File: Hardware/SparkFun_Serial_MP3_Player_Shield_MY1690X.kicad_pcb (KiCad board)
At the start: 2 copper layers, 53.3 x 59.7 mm, 91 parts, among them J1 3.5mm TRRS, J2 Conn_01x04, J4 USB_C_Receptacle, J6 microSD, Q1 BSS138, SW1 SMD_5.2x5.2mm_h2.5mm, U2 MY1690X

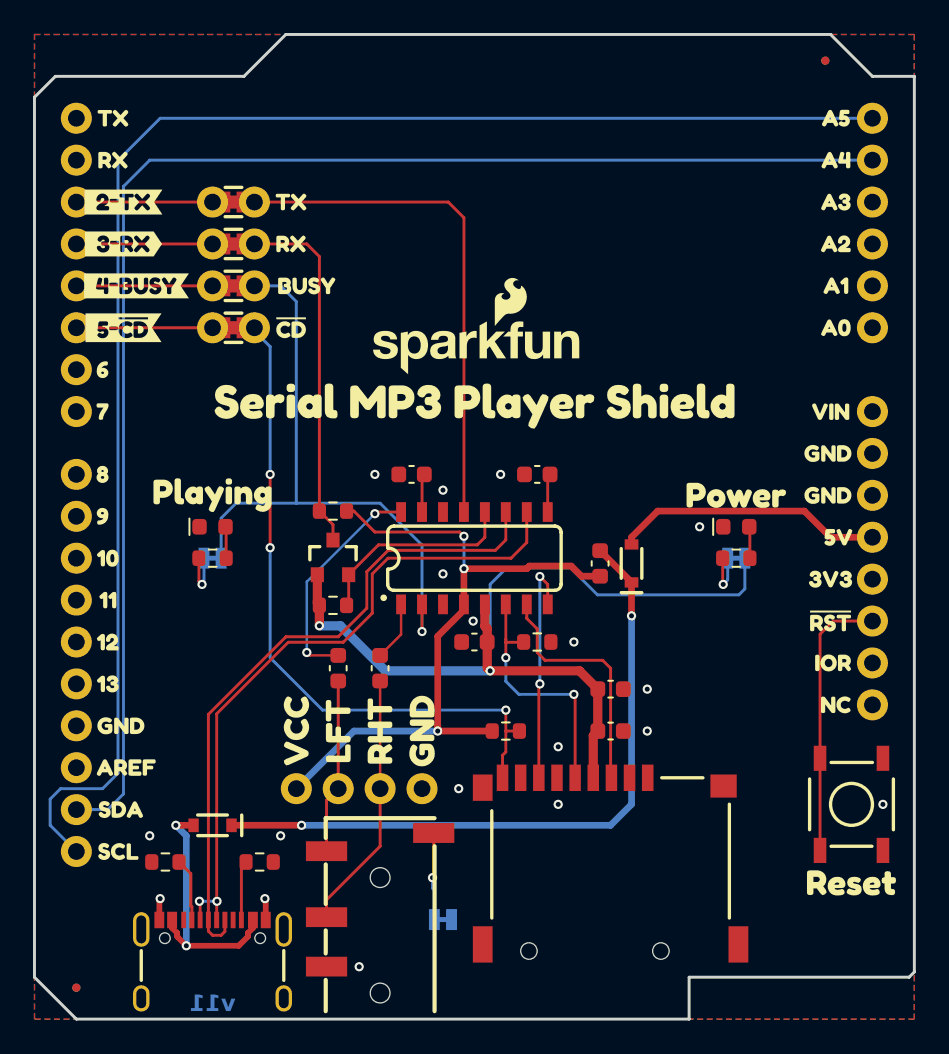
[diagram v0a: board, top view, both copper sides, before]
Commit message: Post review updates.
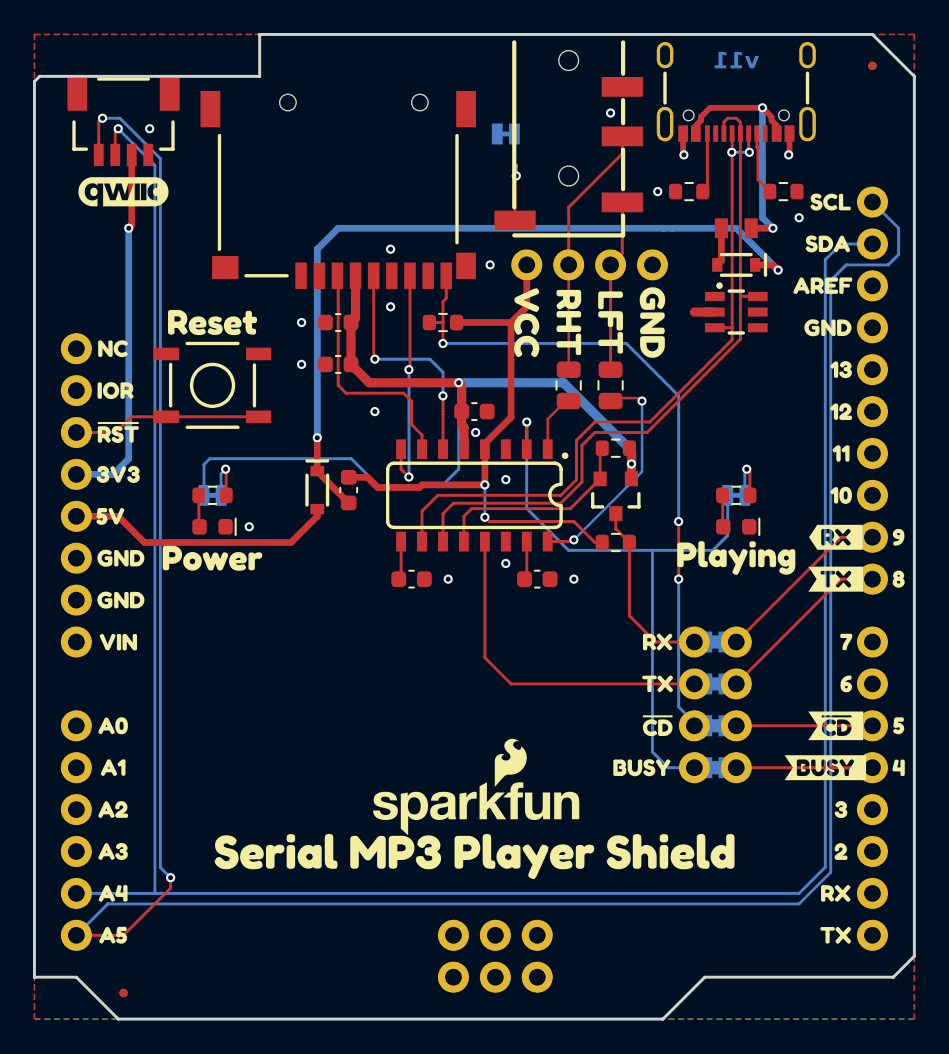
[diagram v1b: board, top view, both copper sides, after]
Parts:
- removed R6: 1k, SparkFun-Resistor:R_0603_1608Metric
- removed kibuzzard-673EA5E2: G***, kibuzzard-673EA5E2
- removed kibuzzard-673EA5F5: G***, kibuzzard-673EA5F5
- removed kibuzzard-673EA5FE: G***, kibuzzard-673EA5FE
- removed kibuzzard-673EAEAD: G***, kibuzzard-673EAEAD
- removed kibuzzard-673EAEB1: G***, kibuzzard-673EAEB1
- removed kibuzzard-6792ACE3: G***, kibuzzard-6792ACE3
- added D5: DT1042-04SO, SparkFun-Semiconductor-Standard:SOT23-6, F.Cu at (177.8, 74.6)
- added F1: 6V/0.5A/1A, SparkFun-Fuse:0805, F.Cu at (177.8, 69.5)
- added G***: LOGO, SparkFun-Aesthetic:qwiic_5.5mm, F.Cu at (140.7, 67.3)
- added J3: Qwiic_RA, SparkFun-Connector:JST_SMD_1.0mm-4_Black, F.Cu at (140.7, 65.1)
- added J5: ISP, SparkFun-Connector:2x03_NoSilk, F.Cu at (163.2, 113.7)
- added kibuzzard-6792ACFA: G***, kibuzzard-6792ACFA, B.Cu at (173.0, 97.2)
- added kibuzzard-6792ACFE: G***, kibuzzard-6792ACFE, B.Cu at (173.0, 94.6)
- added kibuzzard-6792AD08: G***, kibuzzard-6792AD08, B.Cu at (172.1, 102.2)
- added kibuzzard-6792AD10: G***, kibuzzard-6792AD10, B.Cu at (173.0, 99.7)
- added kibuzzard-679D2133: G***, kibuzzard-679D2133, F.Cu at (184.2, 104.8)
- added kibuzzard-679D2139: G***, kibuzzard-679D2139, F.Cu at (184.2, 107.3)
- added kibuzzard-679D21EC: G***, kibuzzard-679D21EC, F.Cu at (183.8, 90.8)
- added kibuzzard-679D21F4: G***, kibuzzard-679D21F4, F.Cu at (187.6, 90.8)
- added kibuzzard-679D21F8: G***, kibuzzard-679D21F8, F.Cu at (187.6, 88.3)
- added kibuzzard-679D21FD: G***, kibuzzard-679D21FD, F.Cu at (183.8, 88.3)
- added kibuzzard-679D221C: G***, kibuzzard-679D221C, F.Cu at (183.8, 99.7)
- added kibuzzard-679D2221: G***, kibuzzard-679D2221, F.Cu at (183.2, 102.2)
- added kibuzzard-679D222D: G***, kibuzzard-679D222D, F.Cu at (187.6, 99.7)
- added kibuzzard-679D2231: G***, kibuzzard-679D2231, F.Cu at (187.6, 102.2)
- C4, C5: value 10uF -> 47uF; footprint SparkFun-Capacitor:C_0603_1608Metric -> SparkFun-Capacitor:C_0805_2012Metric
- JP3, JP4, JP5, JP6: moved to B.Cu
- JP7: value MIC -> SLV
- moved FID2 73.8 mm to (186.1, 59.7), turned to 90 degrees
- moved FID3 73.8 mm to (186.1, 59.7), turned to -90 degrees
- moved FID1 70.7 mm to (140.7, 115.9), turned to 90 degrees
- moved FID4 70.7 mm to (140.7, 115.9), turned to -90 degrees
- moved Ref** 68.2 mm to (186.1, 63.5)
- moved kibuzzard-673EAE53 66.1 mm to (183.8, 112.4)
- moved kibuzzard-673EAF38 66.1 mm to (140.0, 112.4)
- moved kibuzzard-673EAE60 62.4 mm to (183.8, 109.9)
- moved kibuzzard-673EAF33 62.4 mm to (140.0, 109.9)
- moved kibuzzard-673EAF11 58.9 mm to (140.0, 107.3)
- moved kibuzzard-673EAEE5 58.4 mm to (183.5, 67.9)
- moved J4 56.7 mm to (177.8, 64.1), turned to 180 degrees
- moved kibuzzard-673EAF2D 55.6 mm to (140.0, 104.8)
- moved R3 55.3 mm to (180.7, 67.3), turned to 180 degrees
- moved kibuzzard-673EAEDE 54.9 mm to (183.4, 70.5)
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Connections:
- net Net-(U2-DM) renamed /D-
- net Net-(U2-DP) renamed /D+
- B1 pad 3.3V: unconnected-(B1-Pad3.3V) -> 3.3V
- B1 pad A4/SDA: unconnected-(B1-PadA4/SDA) -> SDA
- B1 pad A5/SCL: unconnected-(B1-PadA5/SCL) -> SCL
- B1 pad D2: Net-(JP6-A) -> unconnected-(B1-PadD2)
- B1 pad D3: Net-(B1-*D3) -> unconnected-(B1-*D3-PadD3)
- B1 pad D8: unconnected-(B1-PadD8) -> Net-(JP5-A)
- B1 pad D9: unconnected-(B1-*D9-PadD9) -> Net-(B1-*D9)
- J2 pad 1: VCC -> GND
- J2 pad 4: GND -> VCC
- J4 pad VBUS: VUSB -> Net-(F1-Pad2)
- JP5 pad 1: Net-(B1-*D3) -> Net-(JP5-A)
- JP5 pad 2: MY_RX -> MY_TX
- JP6 pad 1: Net-(JP6-A) -> Net-(B1-*D9)
- JP6 pad 2: MY_TX -> MY_RX
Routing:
- net SCL: track 0.00 -> 150.0 mm, vias 0 -> 2
- net SDA: track 0.00 -> 135.1 mm, vias 0 -> 1
- net unconnected-(B1-PadA5/SCL): track 92.5 -> 0.00 mm
- net unconnected-(B1-PadA4/SDA): track 86.1 -> 0.00 mm
- net 3.3V: track 0.00 -> 22.1 mm, vias 0 -> 1
- net Net-(F1-Pad2): track 0.00 -> 15.9 mm, vias 0 -> 2
- net VUSB: track 15.7 -> 2.33 mm, vias 2 -> 0
- net Net-(JP5-A): track 0.00 -> 10.9 mm
- net Net-(B1-*D9): track 0.00 -> 10.9 mm
- net MY_RX: track 21.8 -> 11.1 mm
- net MY_TX: track 30.9 -> 20.4 mm
- net Net-(JP6-A): track 8.26 -> 0.00 mm
- net Net-(B1-*D3): track 8.26 -> 0.00 mm
- net VCC: track 42.4 -> 36.0 mm, vias 3 -> 2
- net Net-(D2-K): track 40.9 -> 47.2 mm
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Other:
- outline, holes or cut-outs redrawn
